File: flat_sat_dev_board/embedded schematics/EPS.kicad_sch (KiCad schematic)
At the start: 193 parts, among them IC3 PCT2075DP,118, IC4 LT3652IMSE#PBF, IC5 RP2040_QFN56, J12 Foot0, J13 Bypass, J14 ISS Foot, J15 Foot1, J16 Heater, J17 Foot2, J18 Barrel_Jack_Switch, J19 BURN, J20 Foot3, J21 CHARGE, J22 RBF, J24 BM04B-SRSS-TB(LF)(SN), J25 Life Makes Lemonade, J26 Jetson, J27 BM04B-SRSS-TB(LF)(SN), J28 BM04B-SRSS-TB(LF)(SN), J29 CHARGE, J30 CAN1, J31 I2C Multiplexer Breakout, J32 I2C0 Breakout, J34 Screw_Terminal_01x02, J35 Conn_ARM_JTAG_SWD_10, J36 USB_B_Micro, K1 APAN3109, Q10 NDS8434, Q11 MBT2222ADW1T1, Q12 MBT2222ADW1T1, Q2 MMBT2222AT, Q3 IRLML2803, Q4 IRLML2803, Q5 NDS8434, Q6 NDS8434, Q7 IRF7458, Q8 IRF7458, Q9 IRLML2803, SW3 KMR2, SW4 KMR2, U13 1049, U14 R5460N208AA, U15 1049, U16 TPS54226PWPRPWP14_2P31X2P46-L, U17 AD8495, U18 TLVH431 DBZ SOT-23, U19 INA219AxD, U20 INA219AxD, U21 MAX706RESA, U22 ADS1015IDGS, U23 W25Q128JV, U24 MCP25625-E/ML, U25 TPS54226PWPRPWP14_2P31X2P46-L, Y4 Crystal_GND24, Y5 Crystal_GND24

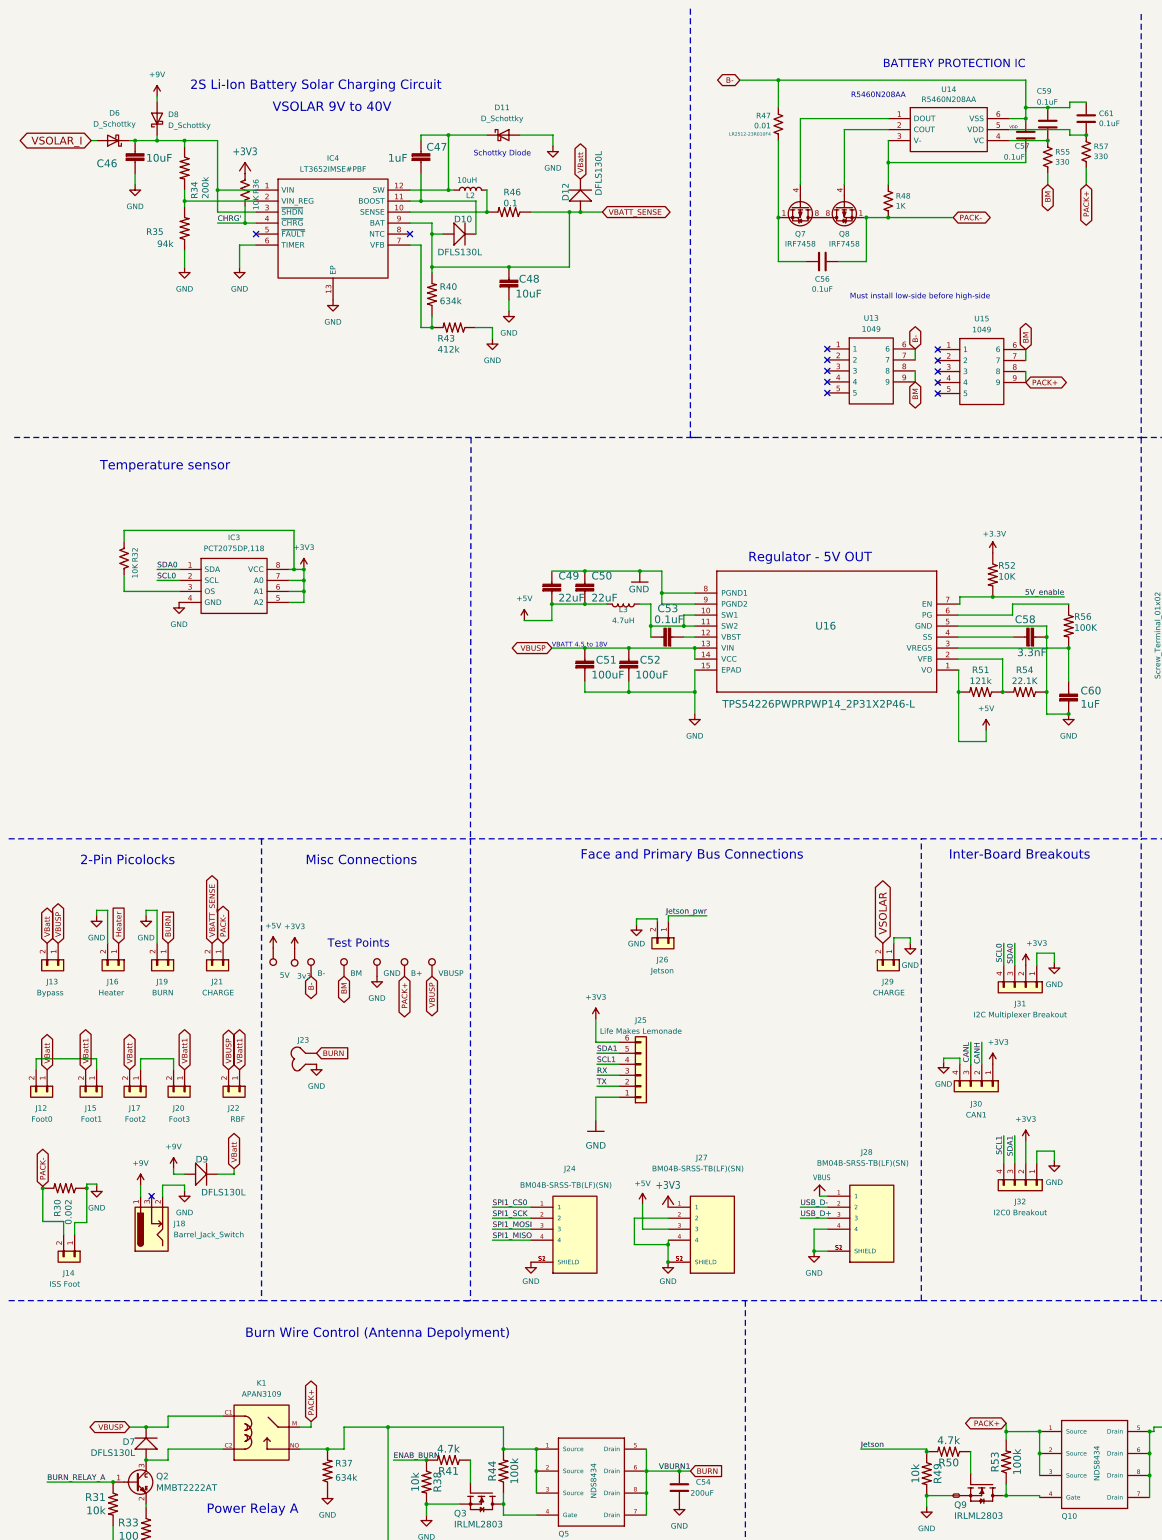
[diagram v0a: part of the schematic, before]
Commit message: Updated all the Diodes!
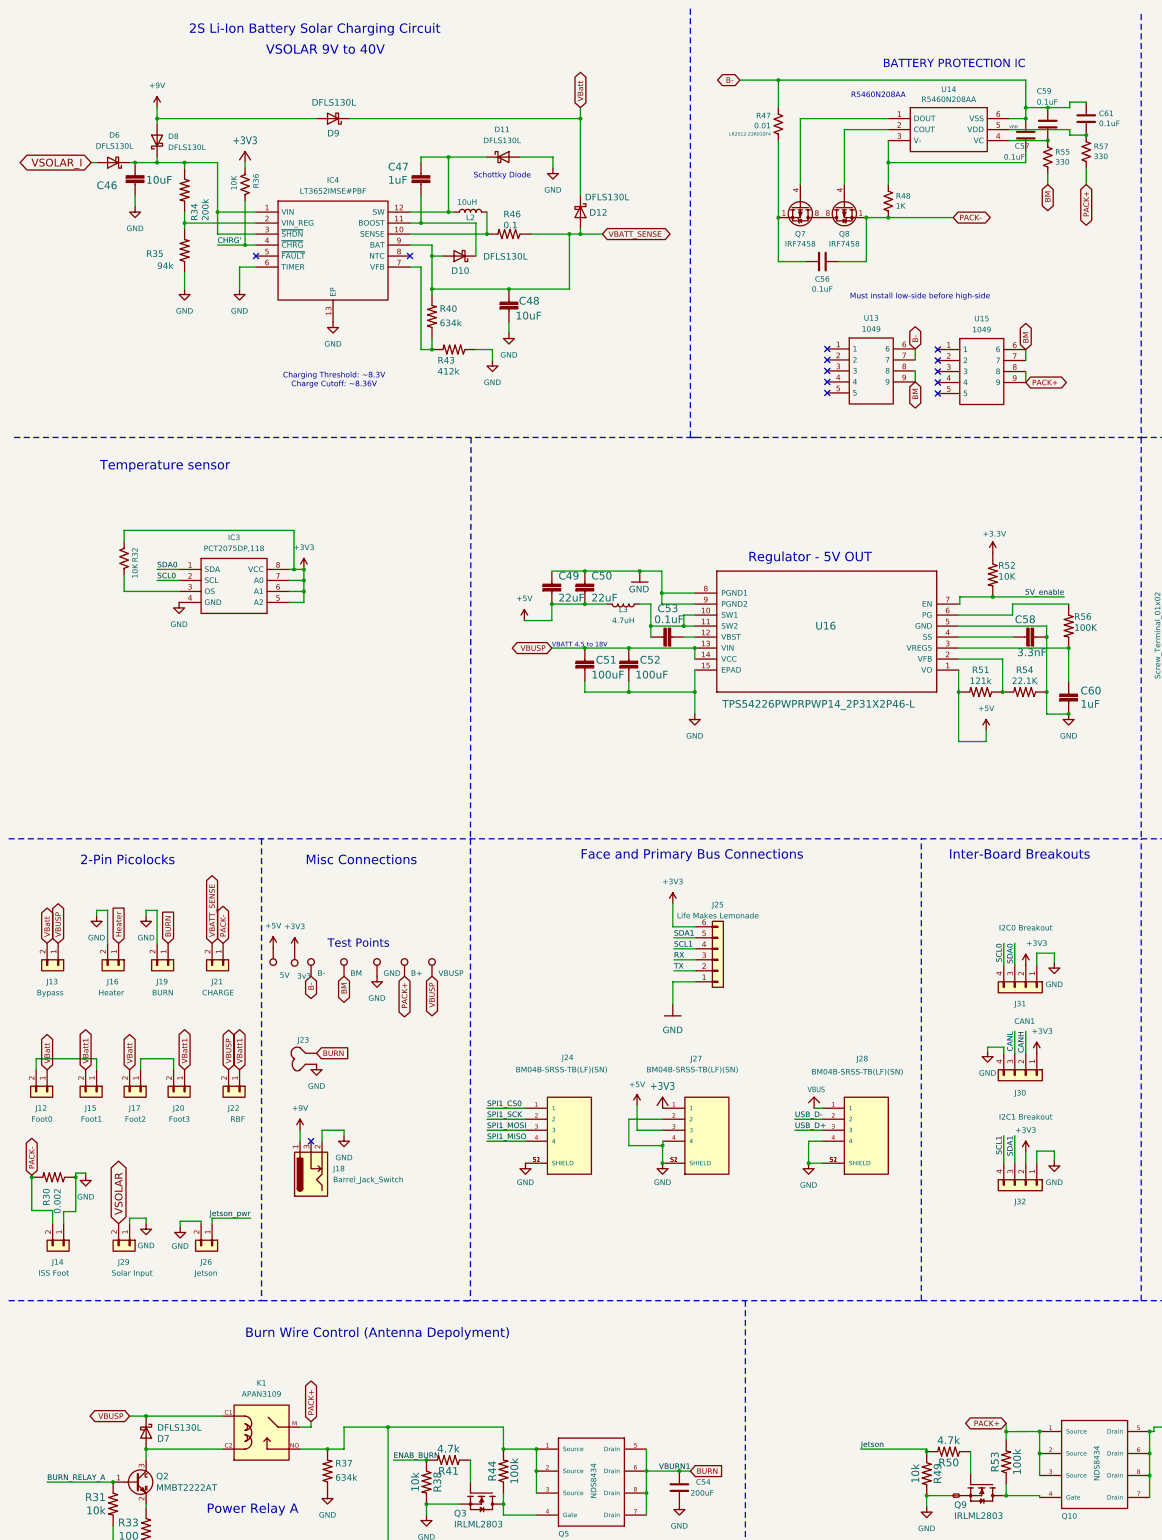
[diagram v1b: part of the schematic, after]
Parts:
- D10, D12, D7, D9: symbol mainboard:DFLS130L -> Device:D_Schottky
- D11, D6, D8: value D_Schottky -> DFLS130L; footprint Diode_SMD:D_SMB -> Diode_SMD:D_PowerDI-123
- J29: value CHARGE -> Solar Input
- J31: value I2C Multiplexer Breakout -> I2C0 Breakout
- J32: value I2C0 Breakout -> I2C1 Breakout
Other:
- note added: "Charging Threshold: ~8.3V Charge Cutoff: ~8.36V"
- moved on the sheet: C46, C47, C48, D11, D6, D8, IC4, J14, J18, J24, J25, J26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
